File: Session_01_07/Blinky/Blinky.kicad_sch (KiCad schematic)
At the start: 8 parts

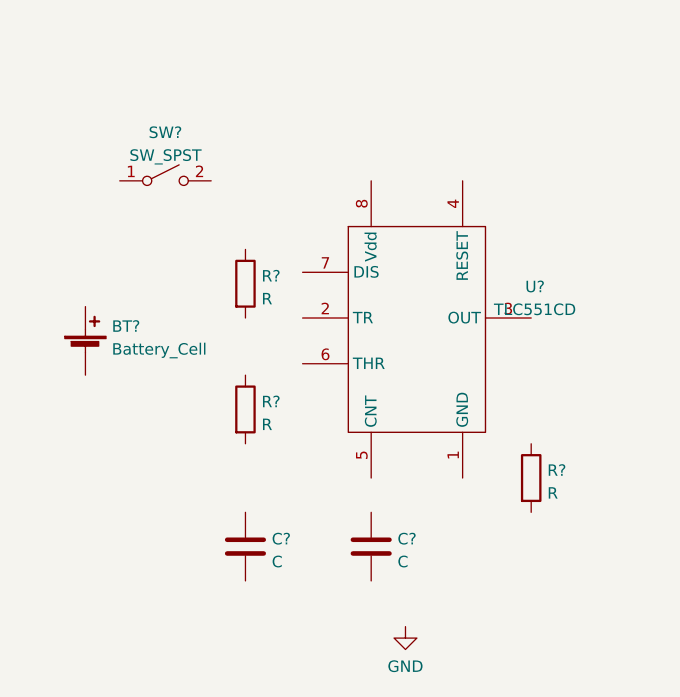
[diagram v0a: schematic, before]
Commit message: Finished the first draft of the work steps
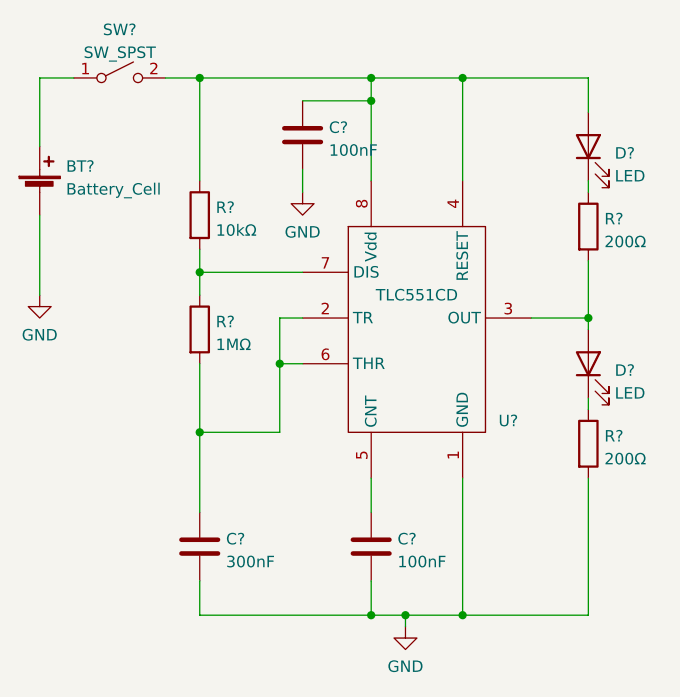
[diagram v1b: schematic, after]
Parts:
- added C?: 100nF, Capacitor_SMD:C_0805_2012Metric_Pad1.18x1.45mm_HandSolder, symbol Device:C
- added D? (x2): LED, LED_SMD:LED_0805_2012Metric_Pad1.15x1.40mm_HandSolder, symbol Device:LED
- added R?: 200Ω, Resistor_SMD:R_0805_2012Metric_Pad1.20x1.40mm_HandSolder, symbol Device:R
- C?: value C -> 100nF; footprint (none) -> Capacitor_SMD:C_0805_2012Metric_Pad1.18x1.45mm_HandSolder
- C?: value C -> 300nF; footprint (none) -> Capacitor_SMD:C_0805_2012Metric_Pad1.18x1.45mm_HandSolder
- R?: value R -> 200Ω; footprint (none) -> Resistor_SMD:R_0805_2012Metric_Pad1.20x1.40mm_HandSolder
- R?: value R -> 10kΩ; footprint (none) -> Resistor_SMD:R_0805_2012Metric_Pad1.20x1.40mm_HandSolder
- R?: value R -> 1MΩ; footprint (none) -> Resistor_SMD:R_0805_2012Metric_Pad1.20x1.40mm_HandSolder
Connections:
- net GND: now also BT?.2 (-), C?.2, C?.2, R?.2, U?.1 (GND), C?.2
- net at C?.1: now also U?.5 (CNT)
- net at U?.2 (TR): now also C?.1, R?.2, U?.6 (THR)
- net at U?.3 (OUT): now also D?.2 (A), R?.2
- net at U?.4 (RESET): now also R?.1, SW?.2 (B), U?.8 (Vdd), C?.1, D?.2 (A)
- net at U?.7 (DIS): now also R?.1, R?.2
- net at R?.1: now also D?.1 (K)
- net at BT?.1 (+): now also SW?.1 (A)
- new net: D?.1 (K), R?.1
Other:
- moved on the sheet: BT?, C?, R?, SW?
